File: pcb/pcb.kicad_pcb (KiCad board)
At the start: 2 copper layers, 71 parts, among them J1 WH, J2 RGB, J3 220, Q1 AO3400A, Q2 AO3400A, Q3 AO3400A, Q4 AO3400A, Q5 AOD452, Q6 DTD114E, Q7 AO3400A, SW1 mode, SW2 bright, T1 ., U1 ATtiny13A-SS, U2 TNY268G, U3 PC817, U4 TL431DBZ, U5 AZ1117-5.0

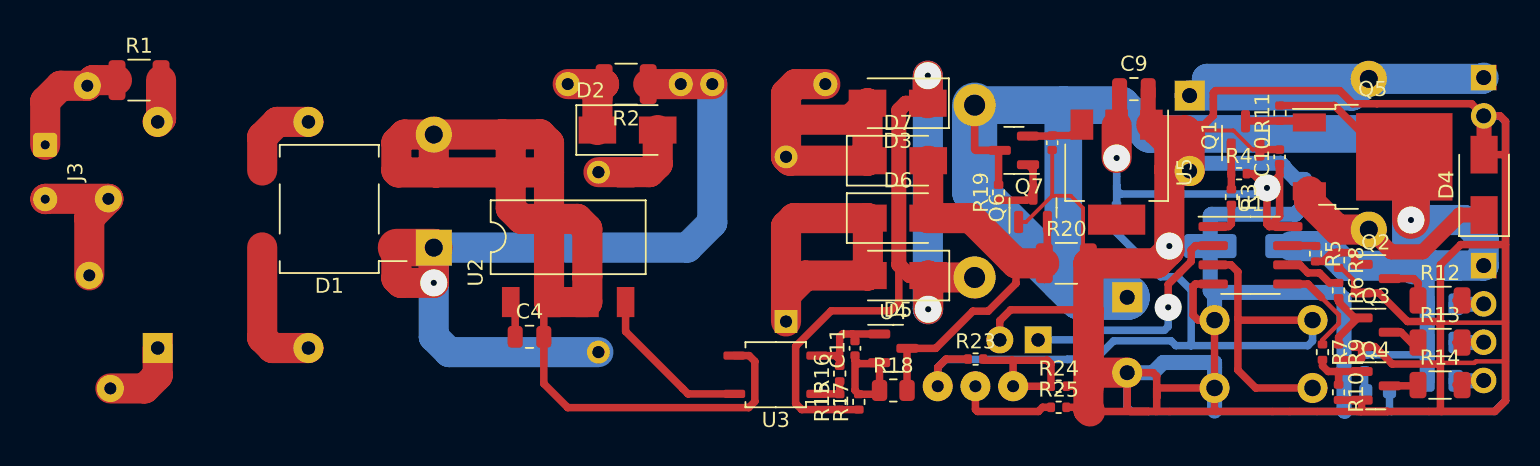
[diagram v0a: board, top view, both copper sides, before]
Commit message: -0.5 cm
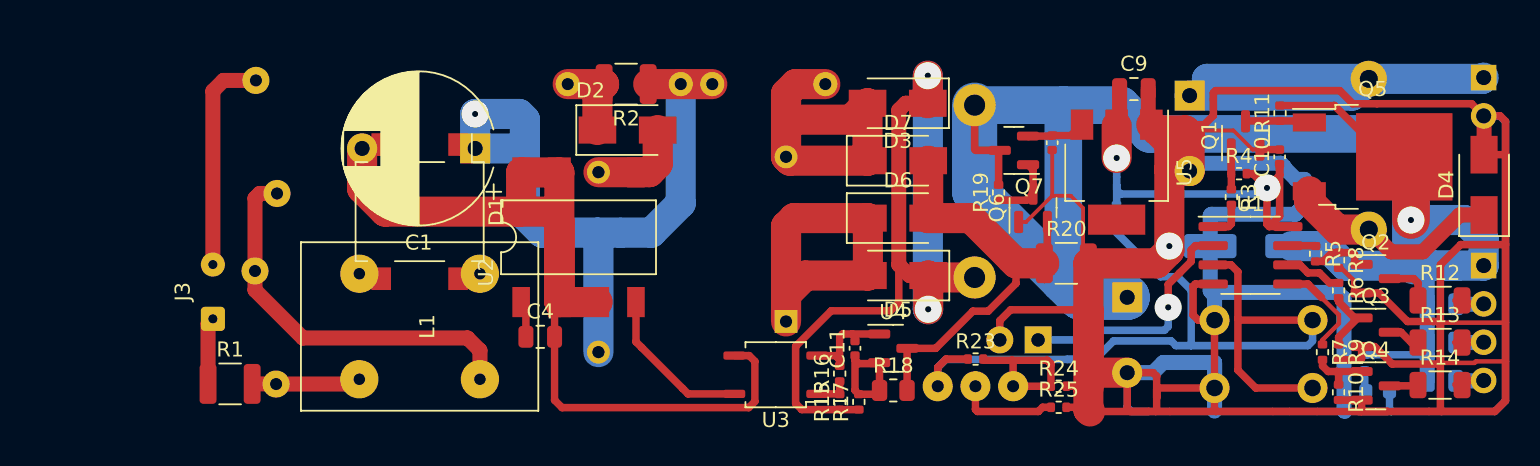
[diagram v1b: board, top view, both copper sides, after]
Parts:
- C1: footprint Capacitor_THT:CP_Radial_D13.0mm_P7.50mm -> Capacitor_THT:CP_Radial_D10.0mm_P7.50mm; moved to F.Cu
- L1: footprint Inductor_THT:Choke_Schaffner_RN212-04-12.5x18.0mm -> local:Input_coil; moved to F.Cu
- moved R1 21.0 mm to (51.3, 48.5)
- moved L1 17.4 mm to (63.9, 44.7), turned to 90 degrees
- moved TH1 17.0 mm to (53.0, 28.4)
- moved J3 16.0 mm to (50.2, 44.2), turned to 90 degrees
- moved RV1 10.8 mm to (53.0, 41.0), turned to -90 degrees
- moved C1 7.13 mm to (67.6, 32.9), turned to 180 degrees
- moved D1 6.00 mm to (63.9, 37.1), turned to -90 degrees
- moved C4 0.71 mm to (71.9, 45.4)
- moved U2 0.69 mm to (74.4, 38.8)
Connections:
- L1 pad 1: Net-(L1-Pad1) -> Net-(TH1-Pad2)
- L1 pad 3: Net-(L1-Pad3) -> Net-(R1-Pad2)
- R1 pad 2: Net-(L1-Pad3) -> Net-(R1-Pad2)
- RV1 pad 1: Net-(J3-Pad2) -> Net-(TH1-Pad2)
- RV1 pad 2: Net-(J3-Pad1) -> Net-(R1-Pad2)
- TH1 pad 2: Net-(L1-Pad1) -> Net-(TH1-Pad2)
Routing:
- net Net-(TH1-Pad2): track 0.00 -> 26.2 mm
- net Net-(C1-Pad2): track 79.1 -> 64.2 mm
- net Net-(C1-Pad1): track 58.6 -> 48.4 mm
- net Net-(D1-Pad4): track 9.35 -> 1.59 mm
- net Net-(R1-Pad2): track 0.00 -> 7.24 mm
- net Net-(L1-Pad1): track 5.32 -> 0.00 mm
- net Net-(J3-Pad2): track 9.81 -> 14.7 mm
- net Net-(D1-Pad3): track 5.70 -> 1.59 mm
- net Net-(J3-Pad1): track 8.24 -> 4.45 mm
- net Net-(L1-Pad3): track 2.86 -> 0.00 mm
